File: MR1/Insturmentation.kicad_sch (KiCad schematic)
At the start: 35 parts, among them J1 Conn_01x01_Pin, J10 Conn_01x01_Pin, J11 Conn_01x01_Pin, J12 Conn_01x10, J2 Conn_01x01_Pin, J9 Conn_01x10, U10 AD40xxBRMZ, U16 LTC6268xS8, U2 LMP7721, U6 ADA4940-1xCP

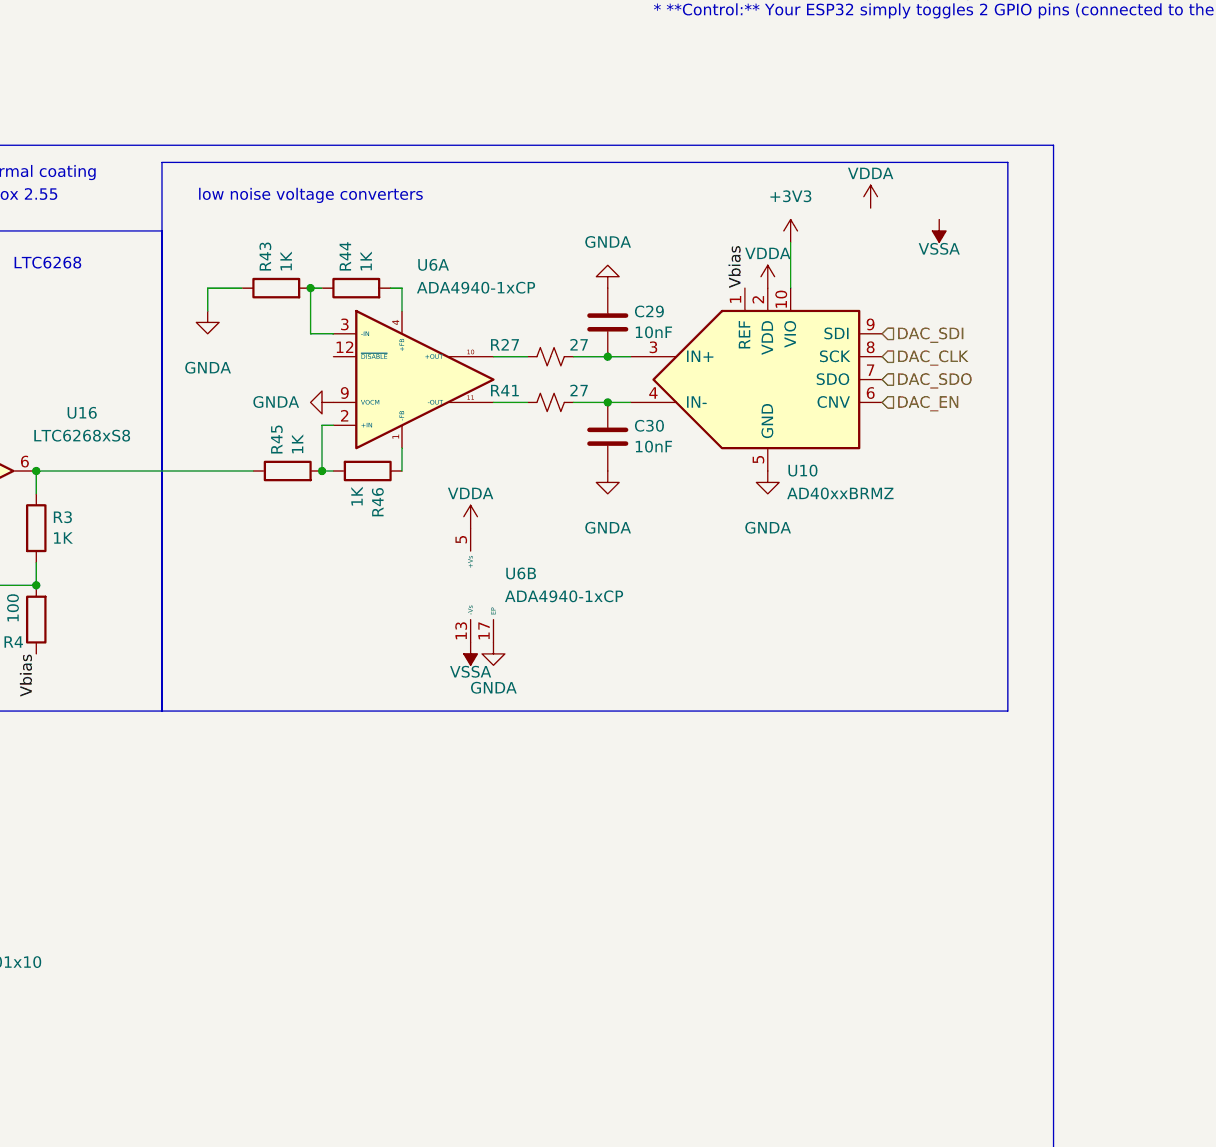
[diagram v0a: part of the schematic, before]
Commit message: Signed-off-by: lokimetasmith <lokimail@gmail.com>
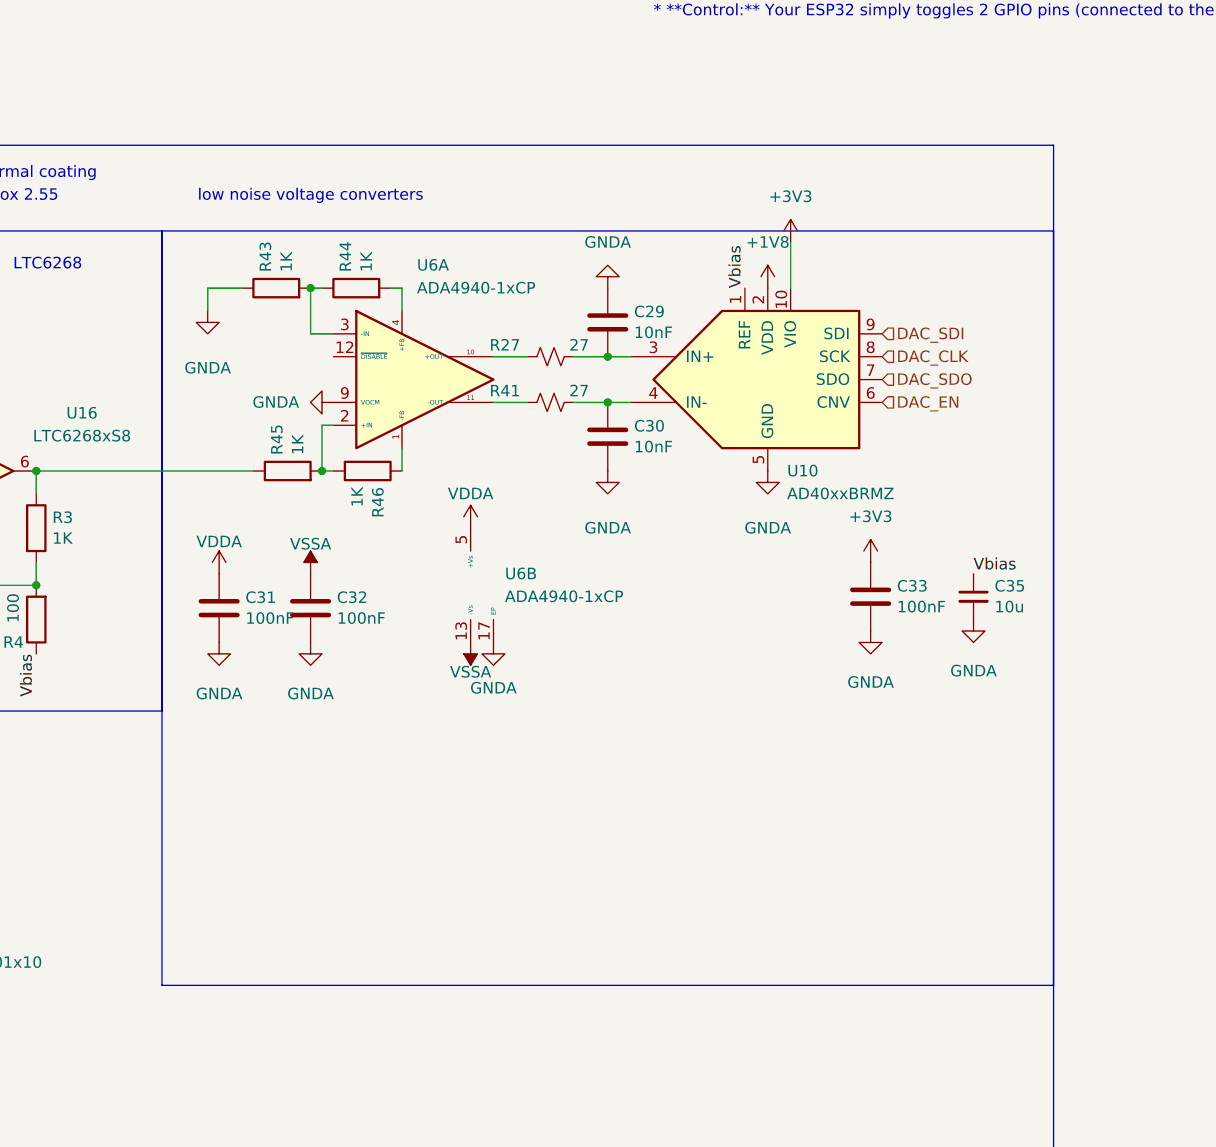
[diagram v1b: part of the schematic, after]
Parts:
- added C31, C32, C33: 100nF, Capacitor_SMD:C_0402_1005Metric, symbol Device:C
- added C35: 10u, Capacitor_SMD:C_0402_1005Metric, symbol Device:C_Small
- U10: MPN (none) -> AD4011BCPZ-RL7; Mouser PN (none) -> 584-AD4011BCPZ-RL7; price (none) -> $21.70
- U16: MPN (none) -> LTC6268IS8#TRPBF; Mouser PN (none) -> 584-LTC6268IS8#TRPBF; price (none) -> $8.40
- U2: MPN (none) -> LMP7721MA/NOPB; price (none) -> $5.13
- U6: MPN (none) -> ADA4940-1ACPZ-RL; Mouser PN (none) -> 584-ADA4940-1ACPZ-R; price (none) -> $4.57
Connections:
- net +3V3: now also C33.1
- net GNDA: now also C31.2, C32.2, C33.2, C35.2
- net VDDA: now also C31.1; no longer U10.2 (VDD)
- net VSSA: now also C32.1
- net Vbias: now also C35.1
- new net +1V8: U10.2 (VDD)
